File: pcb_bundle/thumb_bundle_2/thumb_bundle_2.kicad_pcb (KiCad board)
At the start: 2 copper layers, 99.8 x 99.1 mm, 51 parts

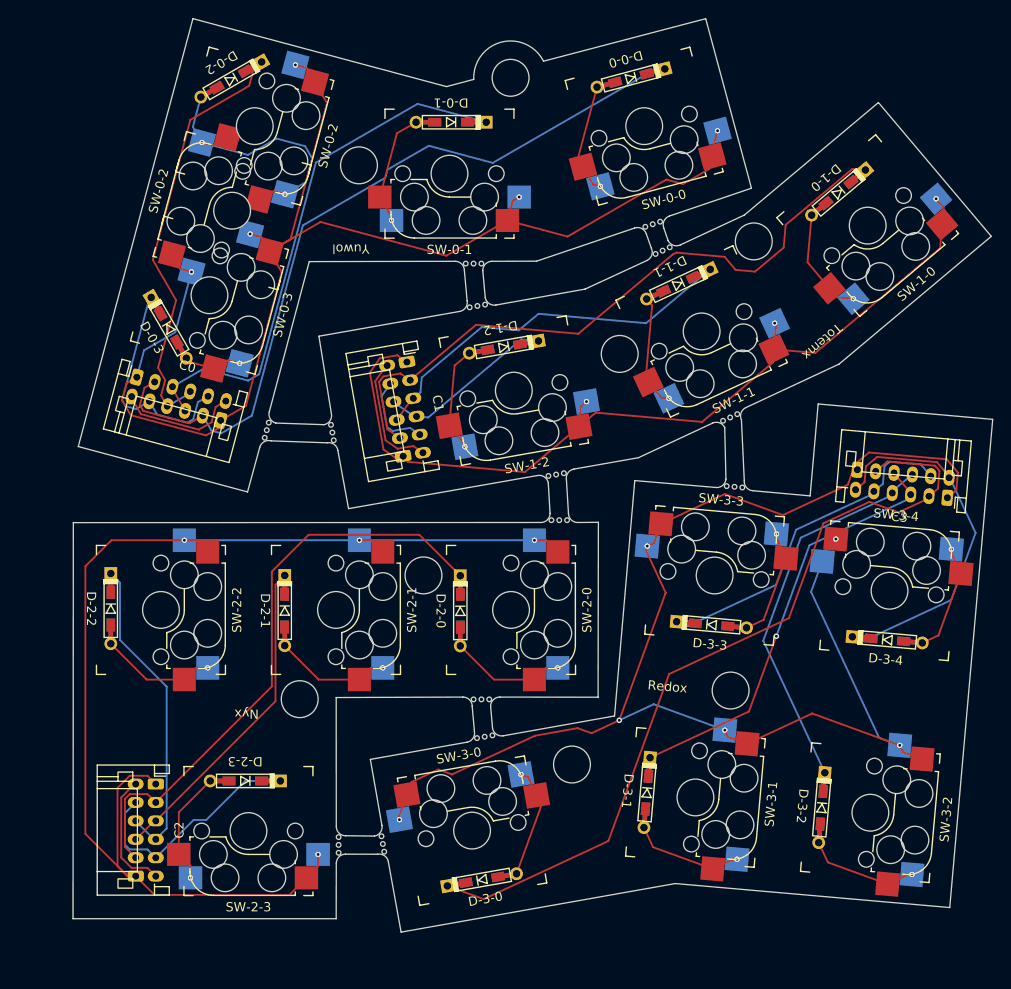
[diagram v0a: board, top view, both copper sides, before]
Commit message: Regenerated bundle
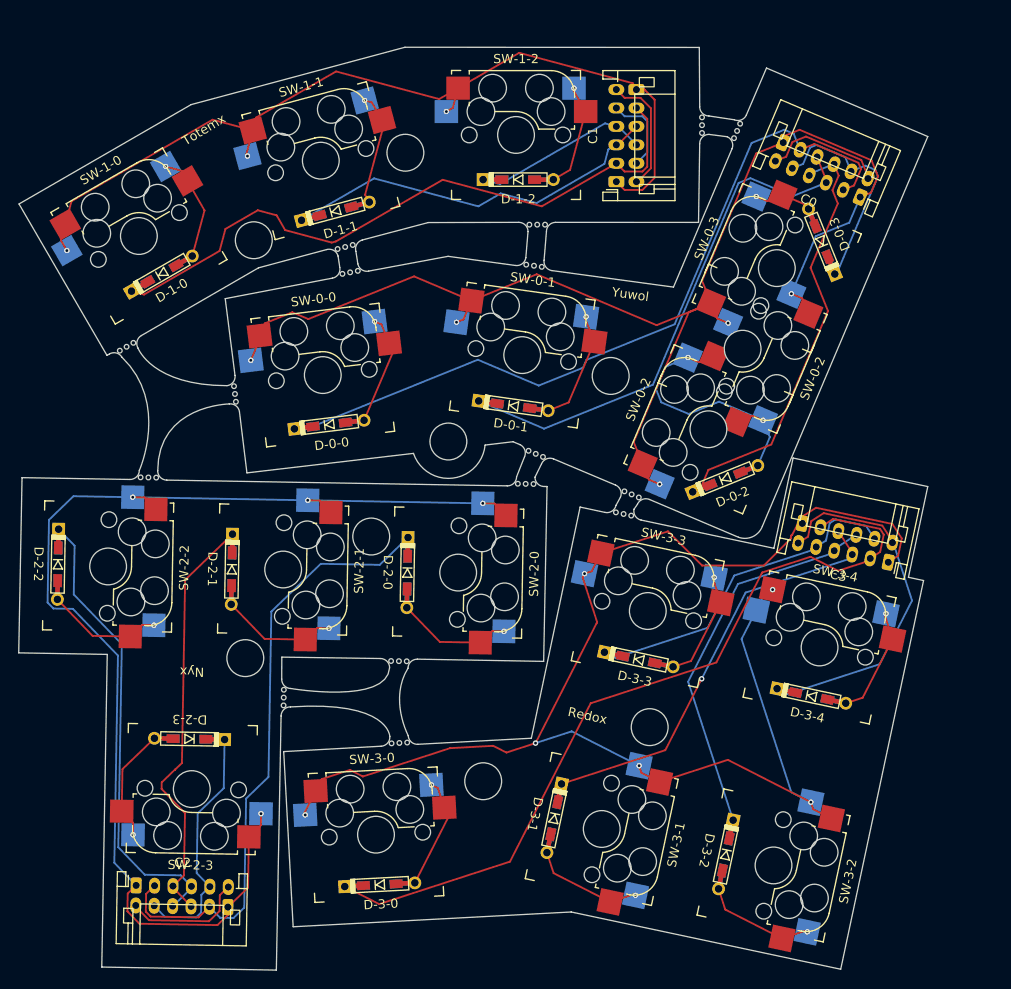
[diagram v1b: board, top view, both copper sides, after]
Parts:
- removed the REF** at (66.0, 98.5)
- removed the REF** at (55.1, 109.8)
- removed the REF** at (65.5, 93.9)
- removed the REF** at (93.0, 71.4)
- removed the REF** at (49.8, 110.0)
- added REF**: MouseBite-Part_2.0x2.0mm_outset_D0.5mm_P0.85mm_3h, Panelization:MouseBite-Part_2.0x2.0mm_outset_D0.5mm_P0.85mm_3h, F.Cu at (80.9, 74.3)
- added REF**: MouseBite-Part_2.0x2.0mm_outset_D0.5mm_P0.85mm_3h, Panelization:MouseBite-Part_2.0x2.0mm_outset_D0.5mm_P0.85mm_3h, F.Cu at (71.5, 67.3)
- added REF**: MouseBite-Part_2.0x2.0mm_outset_D0.5mm_P0.85mm_3h, Panelization:MouseBite-Part_2.0x2.0mm_outset_D0.5mm_P0.85mm_3h, F.Cu at (56.6, 89.8)
- added REF**: MouseBite-Part_2.0x2.0mm_outset_D0.5mm_P0.85mm_3h, Panelization:MouseBite-Part_2.0x2.0mm_outset_D0.5mm_P0.85mm_3h, F.Cu at (43.8, 94.0)
- added REF**: MouseBite-Part_2.0x2.0mm_outset_D0.5mm_P0.85mm_3h, Panelization:MouseBite-Part_2.0x2.0mm_outset_D0.5mm_P0.85mm_3h, F.Cu at (70.3, 71.1)
- added REF**: MouseBite-Part_2.0x2.0mm_outset_D0.5mm_P0.85mm_3h, Panelization:MouseBite-Part_2.0x2.0mm_outset_D0.5mm_P0.85mm_3h, F.Cu at (39.0, 61.0)
- added REF**: MouseBite-Part_2.0x2.0mm_outset_D0.5mm_P0.85mm_3h, Panelization:MouseBite-Part_2.0x2.0mm_outset_D0.5mm_P0.85mm_3h, F.Cu at (82.0, 71.7)
- moved C0 80.9 mm to (106.7, 39.7), turned to 157 degrees
- moved SW-1-0 79.1 mm to (28.4, 43.9), turned to 30 degrees
- moved D-1-0 74.0 mm to (30.9, 48.0), turned to 30 degrees
- moved D-0-3 71.5 mm to (102.5, 44.5), turned to 112 degrees
- moved D-0-2 68.9 mm to (92.0, 70.2), turned to 22 degrees
- moved REF** 66.0 mm to (26.9, 55.7), turned to -150 degrees
- moved SW-0-3 61.7 mm to (97.6, 47.4), turned to 67 degrees
- moved REF** 60.8 mm to (93.5, 32.6), turned to 67 degrees
- moved SW-0-2 59.2 mm to (90.2, 64.9), turned to 67 degrees
- moved SW-0-2 57.4 mm to (93.9, 56.1), turned to -113 degrees
- moved REF** 51.8 mm to (89.2, 31.9), turned to -90 degrees
- moved D-0-0 49.9 mm to (49.0, 64.4), turned to 7 degrees
- moved SW-1-1 45.3 mm to (48.1, 35.7), turned to 15 degrees
- moved REF** 44.2 mm to (29.4, 70.4), turned to -1 degrees
- moved SW-0-0 44.1 mm to (48.3, 59.0), turned to 7 degrees
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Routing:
- net ROW2-2: track 34.7 -> 49.9 mm
- net ROW1-2: track 35.3 -> 45.7 mm
- net COL2: track 134.7 -> 129.9 mm
- net ROW0-2: track 65.0 -> 66.8 mm
- net COL3: track 154.9 -> 156.7 mm
- net ROW3-2: track 26.0 -> 26.8 mm
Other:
- board size 99.8 x 99.1 mm -> 98.7 x 100.2 mm
